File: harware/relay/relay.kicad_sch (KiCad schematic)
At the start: 32 parts, among them J1 Conn_01x04_Socket, J2 Conn_01x04_Socket, J3 Conn_01x04_Socket, J4 Conn_01x04_Socket, K1 SANYOU_SRD_Form_C, K2 SANYOU_SRD_Form_C, K3 SANYOU_SRD_Form_C, K4 SANYOU_SRD_Form_C, U1 GP2S700HCP, U2 L7805, U3 L7805, U4 GP2S700HCP, U5 GP2S700HCP, U6 L7805, U7 GP2S700HCP, U8 L7805

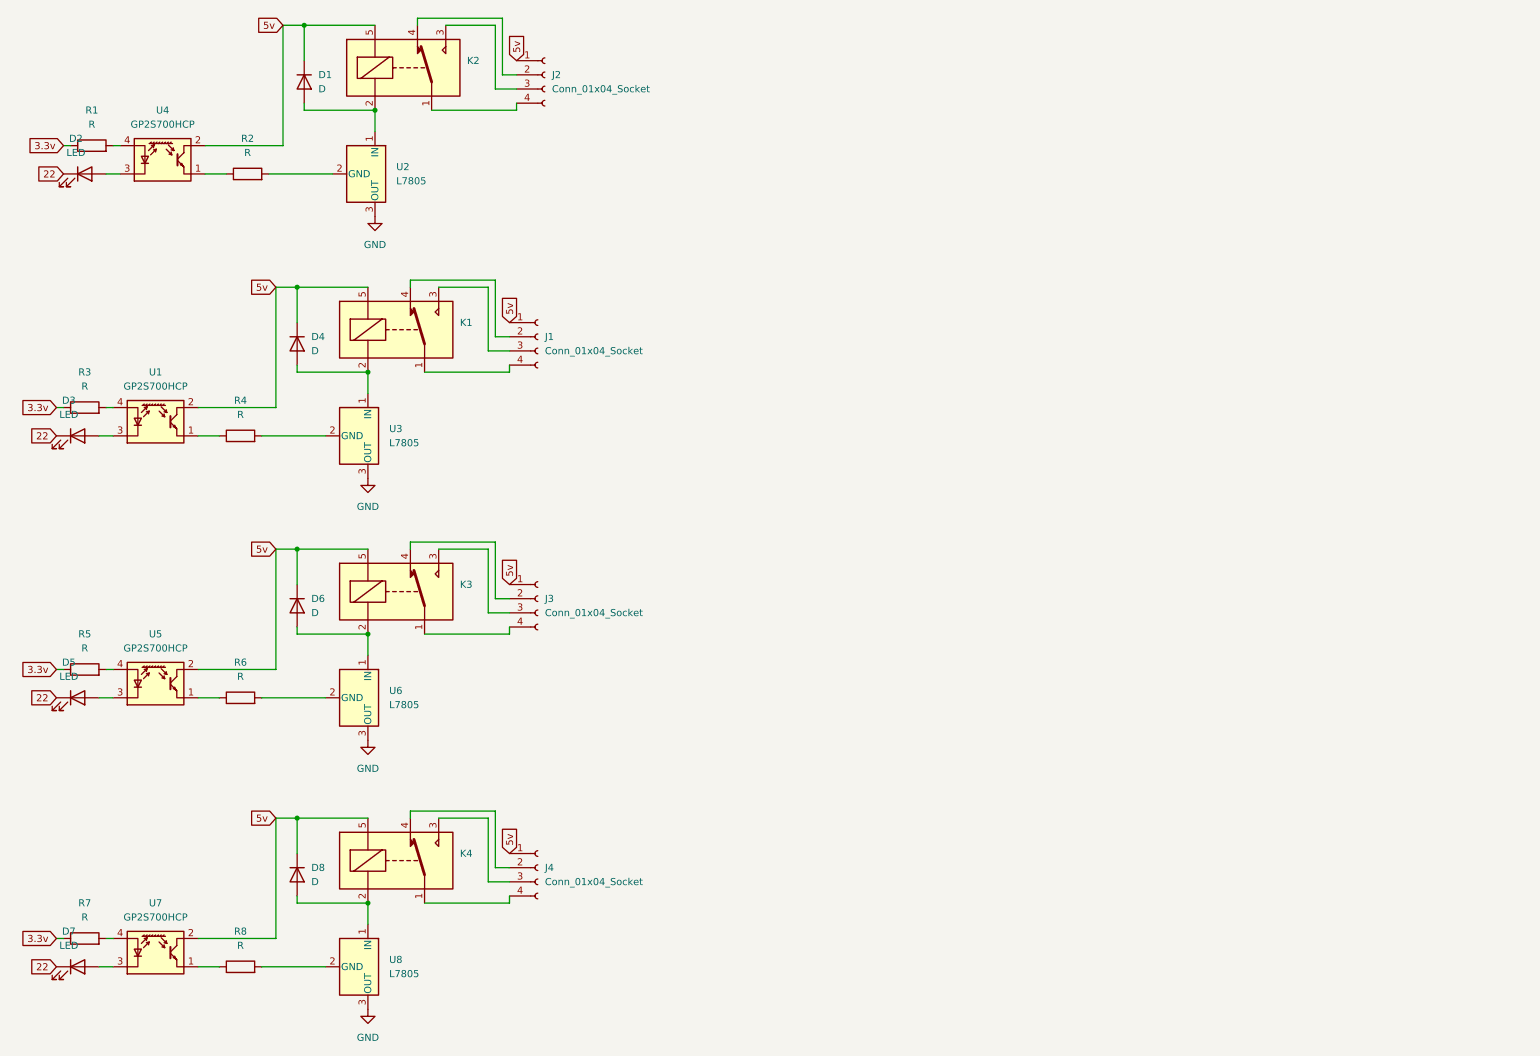
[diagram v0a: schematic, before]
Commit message: commit final
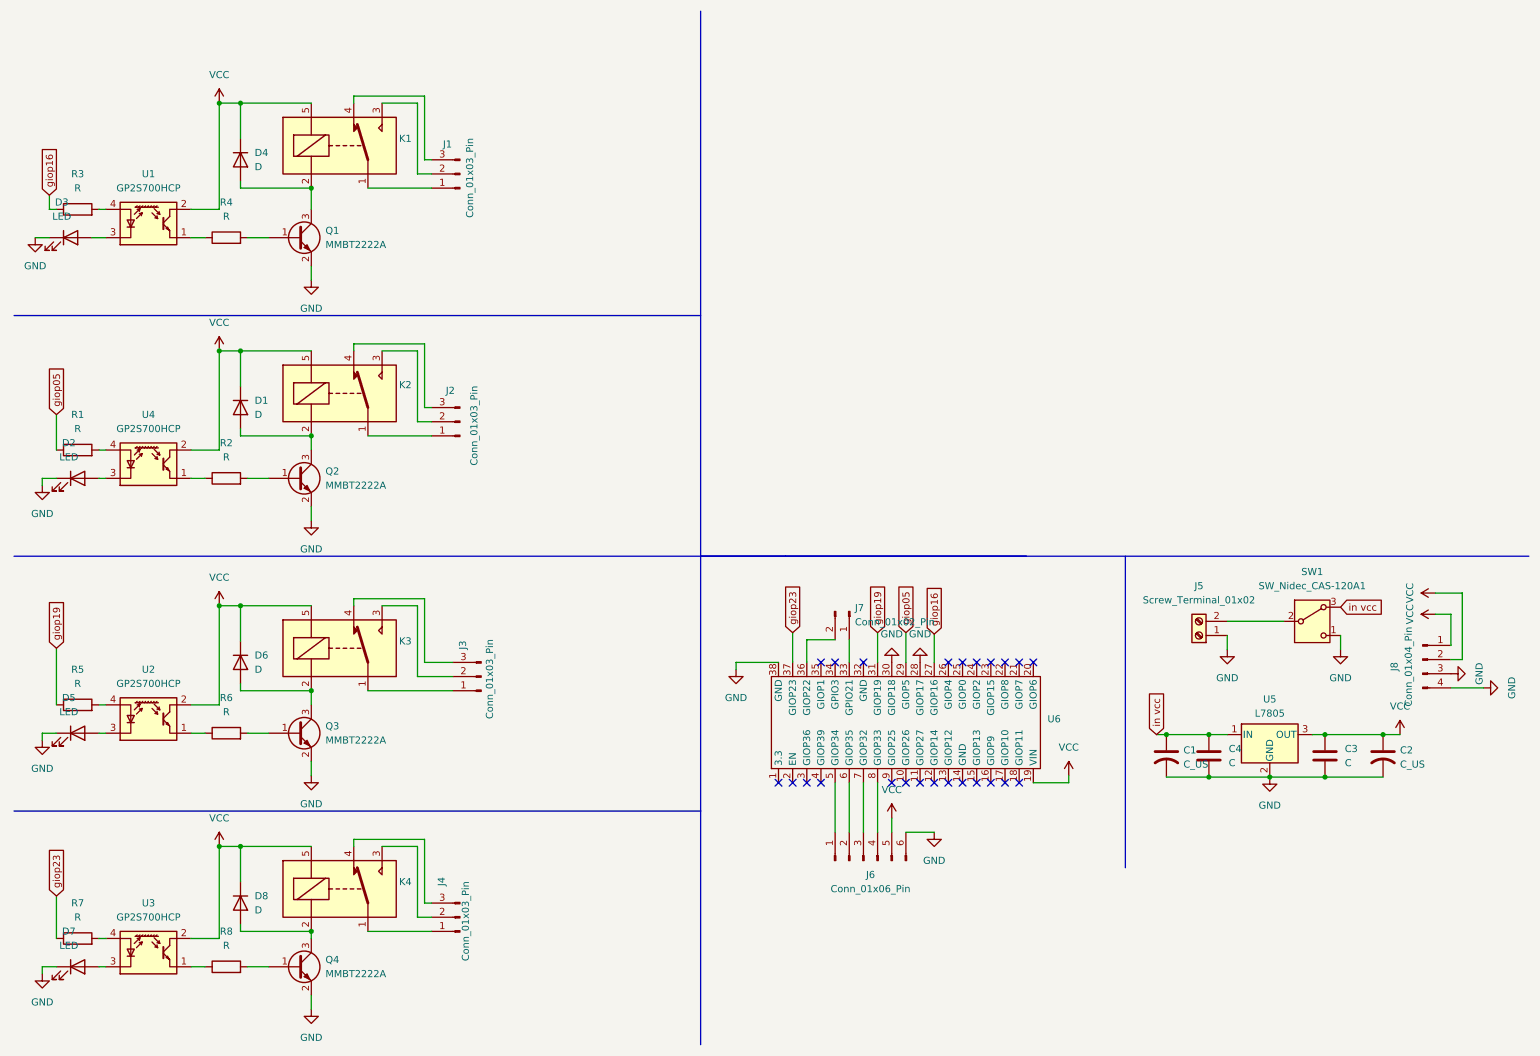
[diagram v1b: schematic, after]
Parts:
- removed J1, J2, J3, J4: Conn_01x04_Socket, TerminalBlock:TerminalBlock_bornier-4_P5.08mm, symbol Connector:Conn_01x04_Socket
- removed U2, U3, U6, U8: L7805, Converter_DCDC:Converter_DCDC_Murata_OKI-78SR_Vertical, symbol Regulator_Linear:L7805
- removed U5, U7: GP2S700HCP, OptoDevice:Sharp_GP2S700HCP, symbol Sensor_Proximity:GP2S700HCP
- added C1, C2: C_US, EESTN5:CAP_ELEC_8x11.5mm, symbol Device:C_US
- added C3, C4: C, EESTN5:CAP_0.1, symbol Device:C
- added J1, J2, J3, J4: Conn_01x03_Pin, TerminalBlock:TerminalBlock_bornier-3_P5.08mm, symbol Connector:Conn_01x03_Pin
- added J5: Screw_Terminal_01x02, TerminalBlock:TerminalBlock_bornier-2_P5.08mm, symbol Connector:Screw_Terminal_01x02
- added J6: Conn_01x06_Pin, Connector_PinHeader_2.00mm:PinHeader_1x06_P2.00mm_Vertical, symbol Connector:Conn_01x06_Pin
- added J7: Conn_01x02_Pin, Connector_PinHeader_2.00mm:PinHeader_1x02_P2.00mm_Vertical, symbol Connector:Conn_01x02_Pin
- added J8: Conn_01x04_Pin, Connector_PinHeader_2.00mm:PinHeader_1x04_P2.00mm_Vertical, symbol Connector:Conn_01x04_Pin
- added Q1, Q2, Q3, Q4: MMBT2222A, Package_TO_SOT_SMD:SOT-23, symbol Transistor_BJT:MMBT2222A
- added SW1: SW_Nidec_CAS-120A1, Connector_PinHeader_2.00mm:PinHeader_1x03_P2.00mm_Vertical, symbol Switch:SW_Nidec_CAS-120A1
- added U2, U3: GP2S700HCP, OptoDevice:Sharp_GP2S700HCP, symbol Sensor_Proximity:GP2S700HCP
- added U5: L7805, Converter_DCDC:Converter_DCDC_RECOM_R-78E-0.5_THT, symbol Regulator_Linear:L7805
- added U6: ~, esp:ESP32S_38_PINES, symbol esp:_1
- R2, R4, R6, R8: footprint (lib_symbols (symbol "Regulator_Linear:L7805" (pin_names (offset 0.254)) (exclude_from_sim no) (in_bom yes) (on_board y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 -> Resistor_SMD:R_0805_2012Metric
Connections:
- net 22 is gone; now on net GND: D2.1 (K), D3.1 (K), D5.1 (K), D7.1 (K)
- net GND: now also C1.2, C2.2, C3.2, C4.2, J5.1 (Pin_1), J6.6 (Pin_6), J8.3 (Pin_3), J8.4 (Pin_4), Q1.2 (E), Q2.2 (E), Q3.2 (E), Q4.2 (E), SW1.1 (C), U5.2 (GND), U6.28 (GIOP17), U6.30 (GIOP18), U6.38 (GND)
- net at D8.2 (A), K4.2: now also Q4.3 (C)
- net at R8.2: now also Q4.1 (B)
- net at K4.1: now also J4.1 (Pin_1)
- net at K4.3: now also J4.2 (Pin_2)
- net at K4.4: now also J4.3 (Pin_3)
- net at R5.2: now also U2.4 (A)
- net at R4.2: now also Q1.1 (B)
- net at D6.2 (A), K3.2: now also Q3.3 (C)
- net at R6.2: now also Q3.1 (B)
- net at D5.2 (A): now also U2.3 (K)
- net at D4.2 (A), K1.2: now also Q1.3 (C)
- net at R6.1: now also U2.1
- net at K3.4: now also J3.3 (Pin_3)
- net at K3.3: now also J3.2 (Pin_2)
- net at K3.1: now also J3.1 (Pin_1)
- net at K1.4: now also J1.3 (Pin_3)
- net at K1.3: now also J1.2 (Pin_2)
- net at K1.1: now also J1.1 (Pin_1)
- net at D1.2 (A), K2.2: now also Q2.3 (C)
- net at R2.2: now also Q2.1 (B)
- net at D7.2 (A): now also U3.3 (K)
- net at R7.2: now also U3.4 (A)
- net at R8.1: now also U3.1
- net at K2.1: now also J2.1 (Pin_1)
- net at K2.3: now also J2.2 (Pin_2)
- net at K2.4: now also J2.3 (Pin_3)
- removed net 3.3v: R1.1, R3.1, R5.1, R7.1
- net 5v renamed VCC
- net VCC: now also C2.1, C3.1, J6.5 (Pin_5), J8.1 (Pin_1), J8.2 (Pin_2), U2.2, U3.2, U5.3 (OUT), U6.19 (VIN)
- new net: J7.1 (Pin_1), U6.33 (GPIO21)
- new net: J7.2 (Pin_2), U6.36 (GIOP22)
- new net: J6.1 (Pin_1), U6.5 (GIOP34)
- new net: J6.2 (Pin_2), U6.6 (GIOP35)
- new net: J6.3 (Pin_3), U6.7 (GIOP32)
- new net: J6.4 (Pin_4), U6.8 (GIOP33)
- new net: J5.2 (Pin_2), SW1.2 (B)
- new net giop05: R1.1, U6.29 (GIOP5)
- new net giop16: R3.1, U6.27 (GIOP16)
- new net giop19: R5.1, U6.31 (GIOP19)
- new net giop23: R7.1, U6.37 (GIOP23)
- new net in vcc: C1.1, C4.1, SW1.3 (A), U5.1 (IN)
- no-connect marks 0 -> 24
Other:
- moved on the sheet: D1, D2, K2, R1, R2, U4
